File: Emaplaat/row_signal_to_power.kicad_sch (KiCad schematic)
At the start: 11 parts, among them IC6 1EDN7550BXTSA1, IC7 74HC1G04GV-Q100H, IC8 1EDN7550BXTSA1, IC9 74LVC1G66GW,125

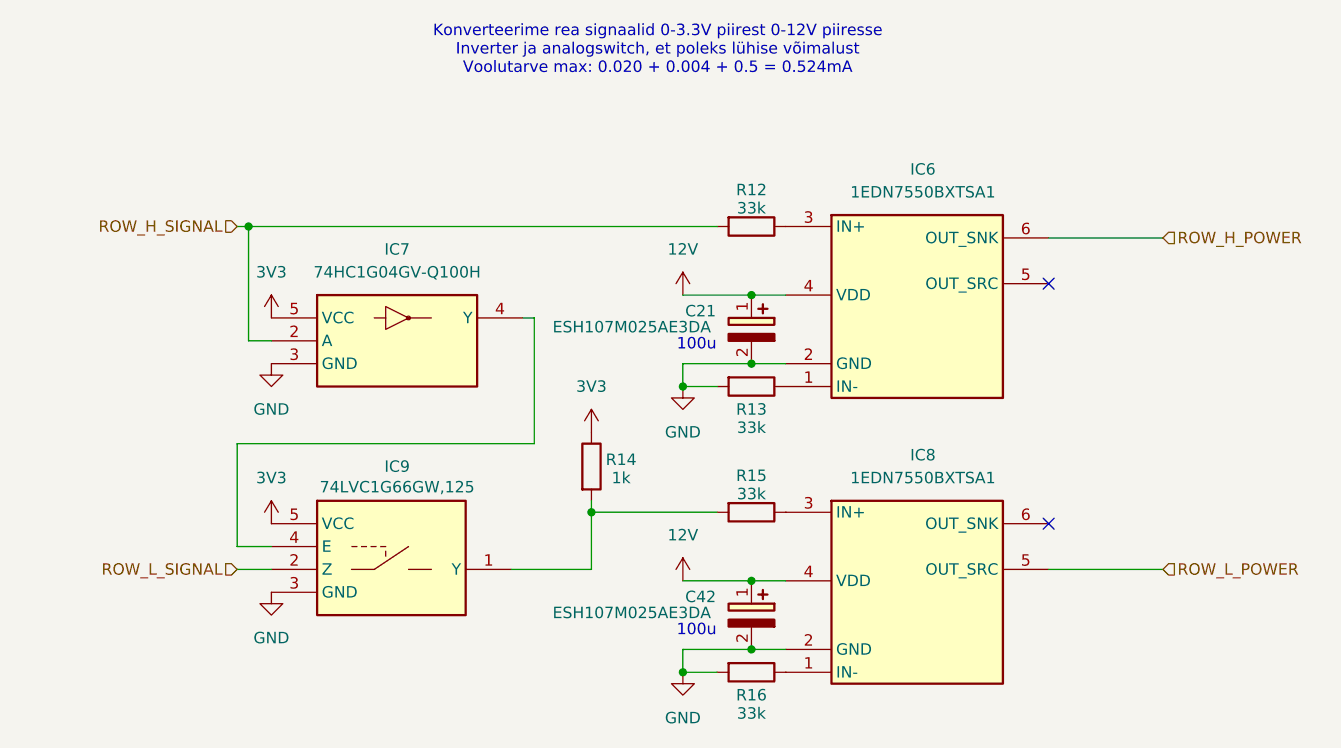
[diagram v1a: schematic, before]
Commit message: v1.5 valmis, juhendajad andsid rohelise tule
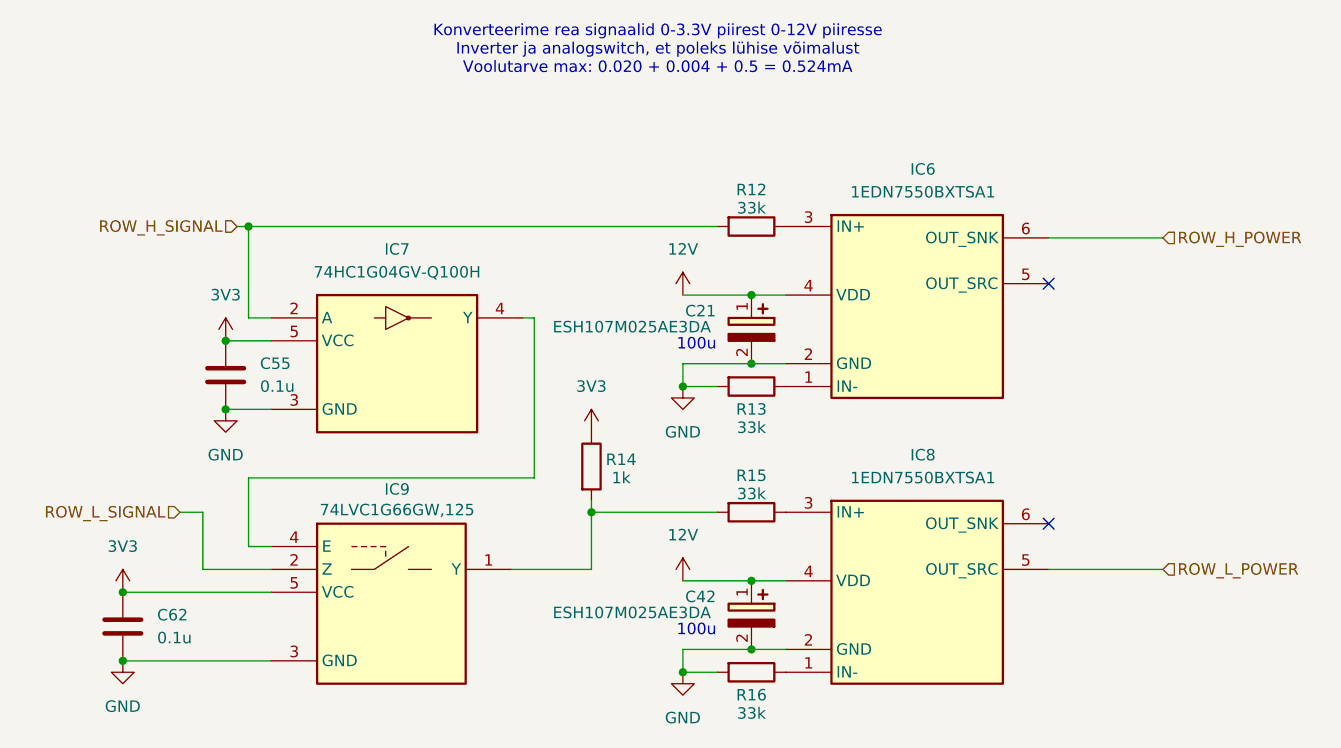
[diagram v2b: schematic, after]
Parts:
- added C55, C62: 0.1u, Capacitor_SMD:C_0603_1608Metric_Pad1.08x0.95mm_HandSolder, symbol Device:C
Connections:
- net 3V3: now also C55.1, C62.1
- net GND: now also C55.2, C62.2
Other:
- moved on the sheet: IC7, IC9
